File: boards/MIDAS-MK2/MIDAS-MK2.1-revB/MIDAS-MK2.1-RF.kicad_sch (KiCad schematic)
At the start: 13 parts, among them J401 SMA, J402 SMA, Q401 Si1016X, U401 RFM96W-433S2, U402 NC7WZ07, U403 MAX-M10S

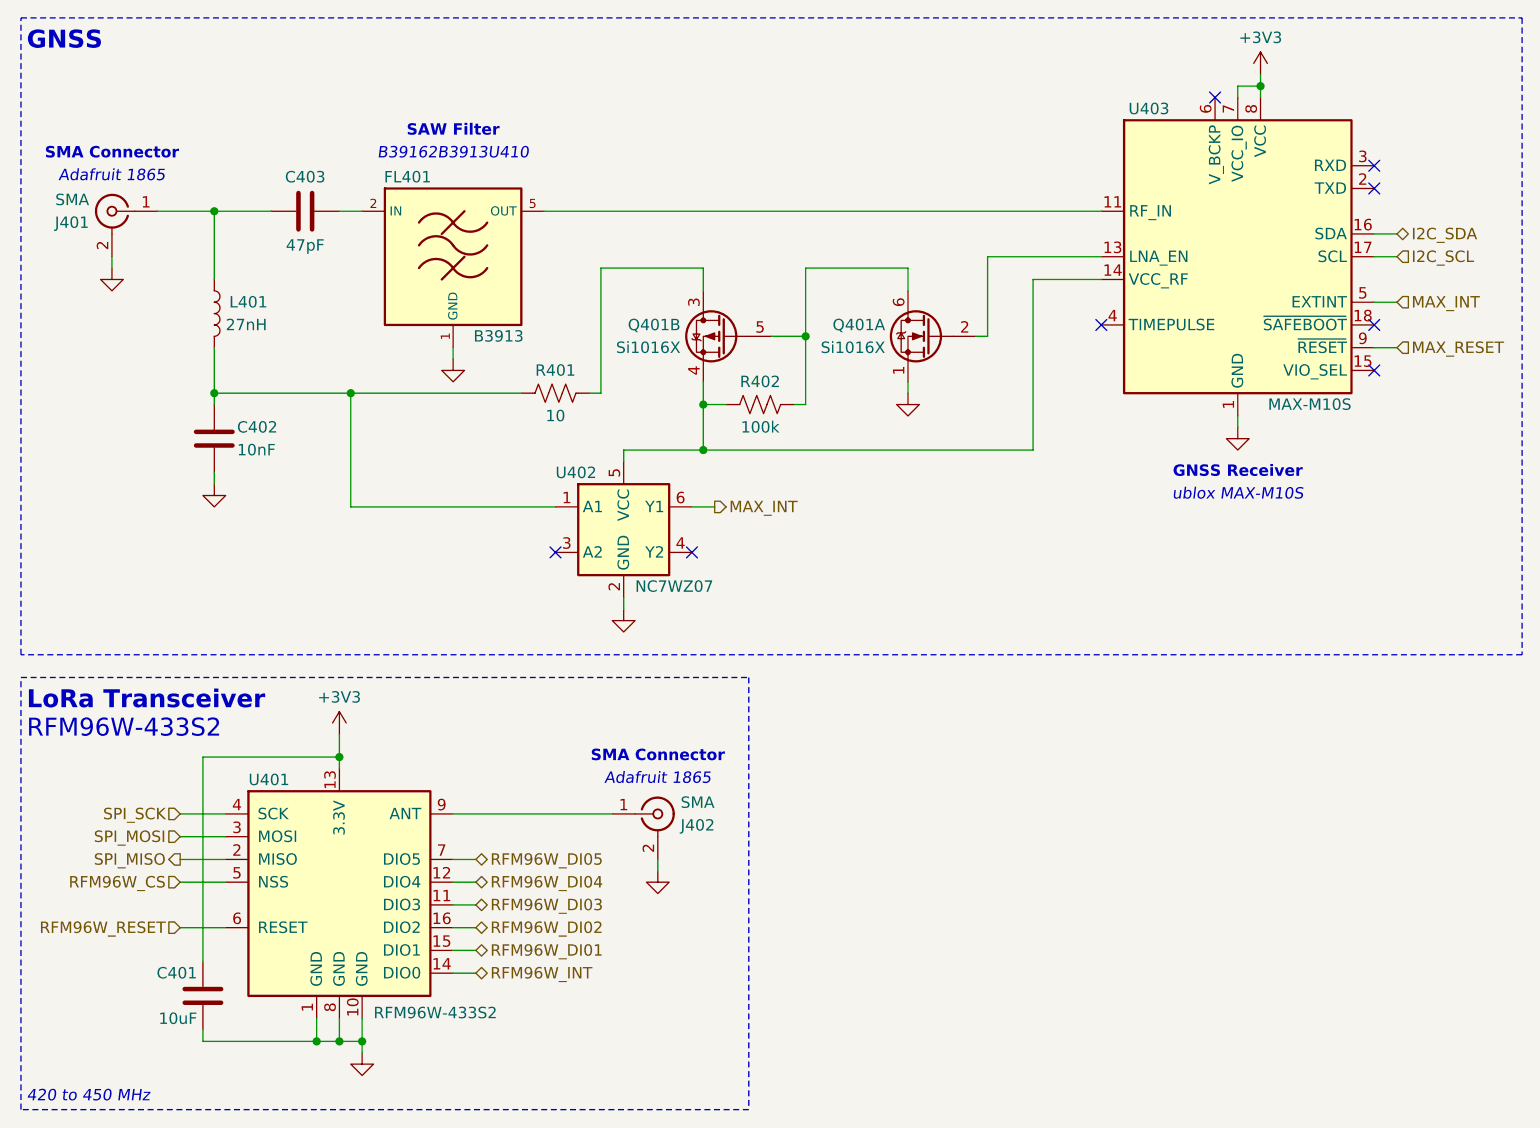
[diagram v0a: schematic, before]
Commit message: DRC error fixes and added accelerometer
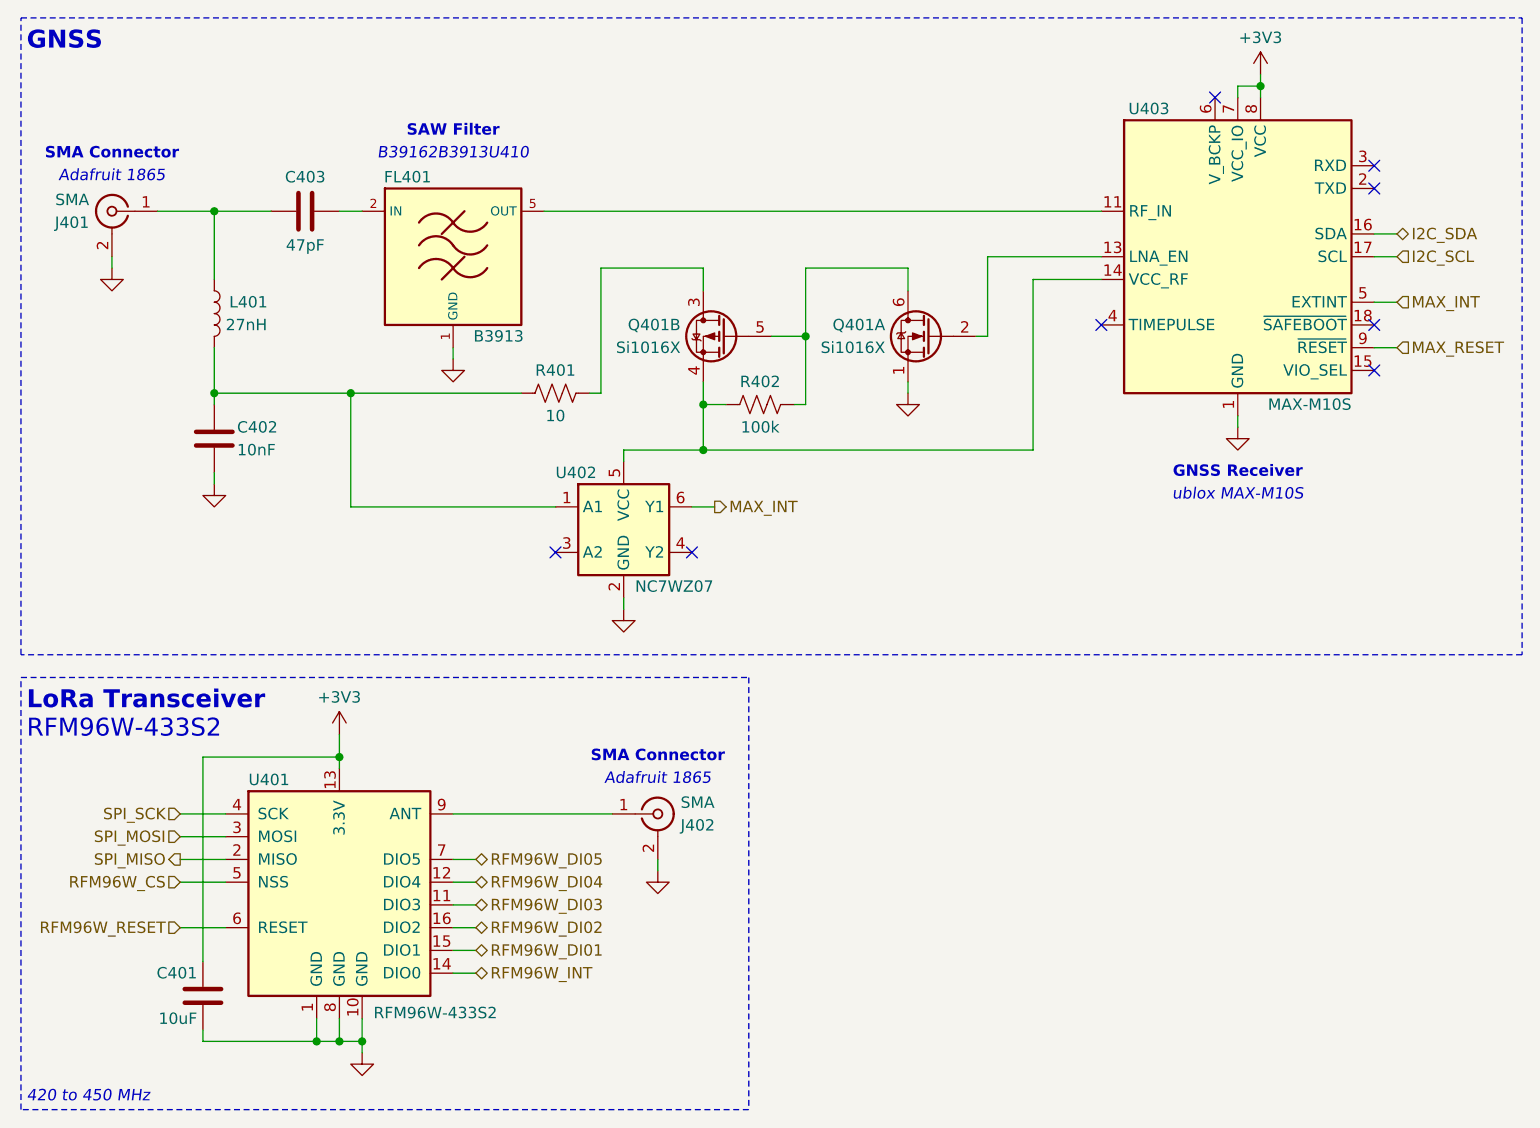
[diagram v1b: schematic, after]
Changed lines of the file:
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@@
 (kicad_sch
-	(version 20231120)
+	(version 20250114)
 	(generator "eeschema")
-	(generator_version "8.0")
+	(generator_version "9.0")
 	(paper "A3")
 	(title_block
@@
 		(comment 4 "Contributors: Thomas McManamen")
 	)
+	(rectangle
+		(start 15.24 15.24)
+		(end 182.88 86.36)
+		(stroke
+			(width 0)
+			(type dash)
+		)
+		(fill
+			(type none)
+		)
+	)
+	(rectangle
+		(start 15.24 88.9)
+		(end 96.52 137.16)
+		(stroke
+			(width 0)
+			(type dash)
+		)
+		(fill
+			(type none)
+		)
+	)
+	(text "B39162B3913U410"
+		(exclude_from_sim no)
+		(at 63.5 30.48 0)
+		(effects
+			(font
+				(size 1.27 1.27)
+				(italic yes)
+			)
+		)
+	)
+	(text "Adafruit 1865"
+		(exclude_from_sim no)
+		(at 86.36 100.33 0)
+		(effects
+			(font
+				(size 1.27 1.27)
+				(italic yes)
+			)
+		)
+	)
+	(text "Adafruit 1865"
+		(exclude_from_sim no)
+		(at 25.4 33.02 0)
+		(effects
+			(font
+				(size 1.27 1.27)
+				(italic yes)
+			)
+		)
+	)
+	(text "420 to 450 MHz"
+		(exclude_from_sim no)
+		(at 15.875 136.525 0)
+		(effects
+			(font
+				(size 1.27 1.27)
+				(italic yes)
+			)
+			(justify left bottom)
+		)
+	)
+	(text "GNSS Receiver"
+		(exclude_from_sim no)
+		(at 151.13 66.04 0)
+		(effects
+			(font
+				(size 1.27 1.27)
+				(thickness 0.254)
+				(bold yes)
+			)
+		)
+	)
+	(text "SMA Connector"
+		(exclude_from_sim no)
+		(at 25.4 30.48 0)
+		(effects
+			(font
+				(size 1.27 1.27)
+				(thickness 0.254)
+				(bold yes)
+			)
+		)
+	)
+	(text "RFM96W-433S2"
+		(exclude_from_sim no)
+		(at 15.875 95.885 0)
+		(effects
+			(font
+				(size 2 2)
+			)
+			(justify left bottom)
+		)
+	)
+	(text "SAW Filter"
+		(exclude_from_sim no)
+		(at 63.5 27.94 0)
+		(effects
+			(font
+				(size 1.27 1.27)
+				(thickness 0.254)
+				(bold yes)
+			)
+		)
+	)
+	(text "SMA Connector"
+		(exclude_from_sim no)
+		(at 86.36 97.79 0)
+		(effects
+			(font
+				(size 1.27 1.27)
+				(thickness 0.254)
+				(bold yes)
+			)
+		)
+	)
+	(text "GNSS"
+		(exclude_from_sim no)
+		(at 15.875 19.05 0)
+		(effects
+			(font
+				(size 2 2)
+				(thickness 0.4)
+				(bold yes)
+			)
+			(justify left bottom)
+		)
+	)
+	(text "ublox MAX-M10S"
+		(exclude_from_sim no)
+		(at 151.13 68.58 0)
+		(effects
+			(font
+				(size 1.27 1.27)
+				(italic yes)
+			)
+		)
+	)
+	(text "LoRa Transceiver"
+		(exclude_from_sim no)
+		(at 15.875 92.71 0)
+		(effects
+			(font
+				(size 2 2)
+				(bold yes)
+			)
+			(justify left bottom)
+		)
+	)
 	(junction
 		(at 91.44 58.42)
@@
 		)
 	)
-	(rectangle
-		(start 15.24 15.24)
-		(end 182.88 86.36)
-		(stroke
-			(width 0)
-			(type dash)
-		)
-		(fill
-			(type none)
-		)
-	)
-	(rectangle
-		(start 15.24 88.9)
-		(end 96.52 137.16)
-		(stroke
-			(width 0)
-			(type dash)
-		)
-		(fill
-			(type none)
-		)
-	)
-	(text "B39162B3913U410"
-		(exclude_from_sim no)
-		(at 63.5 30.48 0)
-		(effects
-			(font
-				(size 1.27 1.27)
-				(italic yes)
-			)
-		)
-	)
-	(text "Adafruit 1865"
-		(exclude_from_sim no)
-		(at 86.36 100.33 0)
-		(effects
-			(font
-				(size 1.27 1.27)
-				(italic yes)
-			)
-		)
-	)
-	(text "Adafruit 1865"
-		(exclude_from_sim no)
-		(at 25.4 33.02 0)
-		(effects
-			(font
-				(size 1.27 1.27)
-				(italic yes)
-			)
-		)
-	)
-	(text "420 to 450 MHz"
-		(exclude_from_sim no)
-		(at 15.875 136.525 0)
-		(effects
-			(font
-				(size 1.27 1.27)
-				(italic yes)
-			)
-			(justify left bottom)
-		)
-	)
-	(text "GNSS Receiver"
-		(exclude_from_sim no)
-		(at 151.13 66.04 0)
-		(effects
-			(font
-				(size 1.27 1.27)
-				(thickness 0.254)
-				(bold yes)
-			)
-		)
-	)
-	(text "SMA Connector"
-		(exclude_from_sim no)
-		(at 25.4 30.48 0)
-		(effects
-			(font
-				(size 1.27 1.27)
-				(thickness 0.254)
-				(bold yes)
-			)
-		)
-	)
-	(text "RFM96W-433S2"
-		(exclude_from_sim no)
-		(at 15.875 95.885 0)
-		(effects
-			(font
-				(size 2 2)
-			)
-			(justify left bottom)
-		)
-	)
-	(text "SAW Filter"
-		(exclude_from_sim no)
-		(at 63.5 27.94 0)
-		(effects
-			(font
-				(size 1.27 1.27)
-				(thickness 0.254)
-				(bold yes)
-			)
-		)
-	)
-	(text "SMA Connector"
-		(exclude_from_sim no)
-		(at 86.36 97.79 0)
-		(effects
-			(font
-				(size 1.27 1.27)
-				(thickness 0.254)
-				(bold yes)
-			)
-		)
-	)
-	(text "GNSS"
-		(exclude_from_sim no)
-		(at 15.875 19.05 0)
-		(effects
-			(font
-				(size 2 2)
-				(thickness 0.4)
-				(bold yes)
-			)
-			(justify left bottom)
-		)
-	)
-	(text "ublox MAX-M10S"
-		(exclude_from_sim no)
-		(at 151.13 68.58 0)
-		(effects
-			(font
-				(size 1.27 1.27)
-				(italic yes)
-			)
-		)
-	)
-	(text "LoRa Transceiver"
-		(exclude_from_sim no)
-		(at 15.875 92.71 0)
-		(effects
-			(font
-				(size 2 2)
-				(bold yes)
-			)
-			(justify left bottom)
-		)
-	)
 	(hierarchical_label "SPI_SCK"
 		(shape input)
 		(at 33.02 104.14 180)
-		(fields_autoplaced yes)
 		(effects
 			(font
@@
 		(shape output)
 		(at 33.02 109.22 180)
-		(fields_autoplaced yes)
 		(effects
 			(font
@@
 		(shape input)
 		(at 168.91 52.07 0)
-		(fields_autoplaced yes)
 		(effects
 			(font
@@
 		(shape input)
 		(at 168.91 46.99 0)
-		(fields_autoplaced yes)
 		(effects
 			(font
@@
 		(shape bidirectional)
 		(at 66.04 109.22 0)
-		(fields_autoplaced yes)
 		(effects
 			(font
@@
 		(shape input)
 		(at 33.02 116.84 180)
-		(fields_autoplaced yes)
 		(effects
 			(font
@@
 		(shape input)
 		(at 33.02 111.76 180)
-		(fields_autoplaced yes)
 		(effects
 			(font
@@
 		(shape output)
 		(at 92.71 69.85 0)
-		(fields_autoplaced yes)
 		(effects
 			(font
@@
 		(shape bidirectional)
 		(at 66.04 121.92 0)
-		(fields_autoplaced yes)
 		(effects
 			(font
@@
 		(shape bidirectional)
 		(at 168.91 39.37 0)
-		(fields_autoplaced yes)
 		(effects
 			(font
@@
 		(shape bidirectional)
 		(at 66.04 111.76 0)
-		(fields_autoplaced yes)
 		(effects
 			(font
@@
 		(shape input)
 		(at 33.02 106.68 180)
-		(fields_autoplaced yes)
 		(effects
 			(font
@@
 		(shape bidirectional)
 		(at 66.04 119.38 0)
-		(fields_autoplaced yes)
 		(effects
 			(font
@@
 		(shape bidirectional)
 		(at 66.04 114.3 0)
-		(fields_autoplaced yes)
 		(effects
 			(font
@@
 		(shape bidirectional)
 		(at 66.04 116.84 0)
-		(fields_autoplaced yes)
 		(effects
 			(font
@@
 		(shape input)
 		(at 168.91 41.91 0)
-		(fields_autoplaced yes)
-		(effects
-			(font
+		(effects
+			(font
